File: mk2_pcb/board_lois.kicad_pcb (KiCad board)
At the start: 2 copper layers, 99 x 90 mm, 38 parts

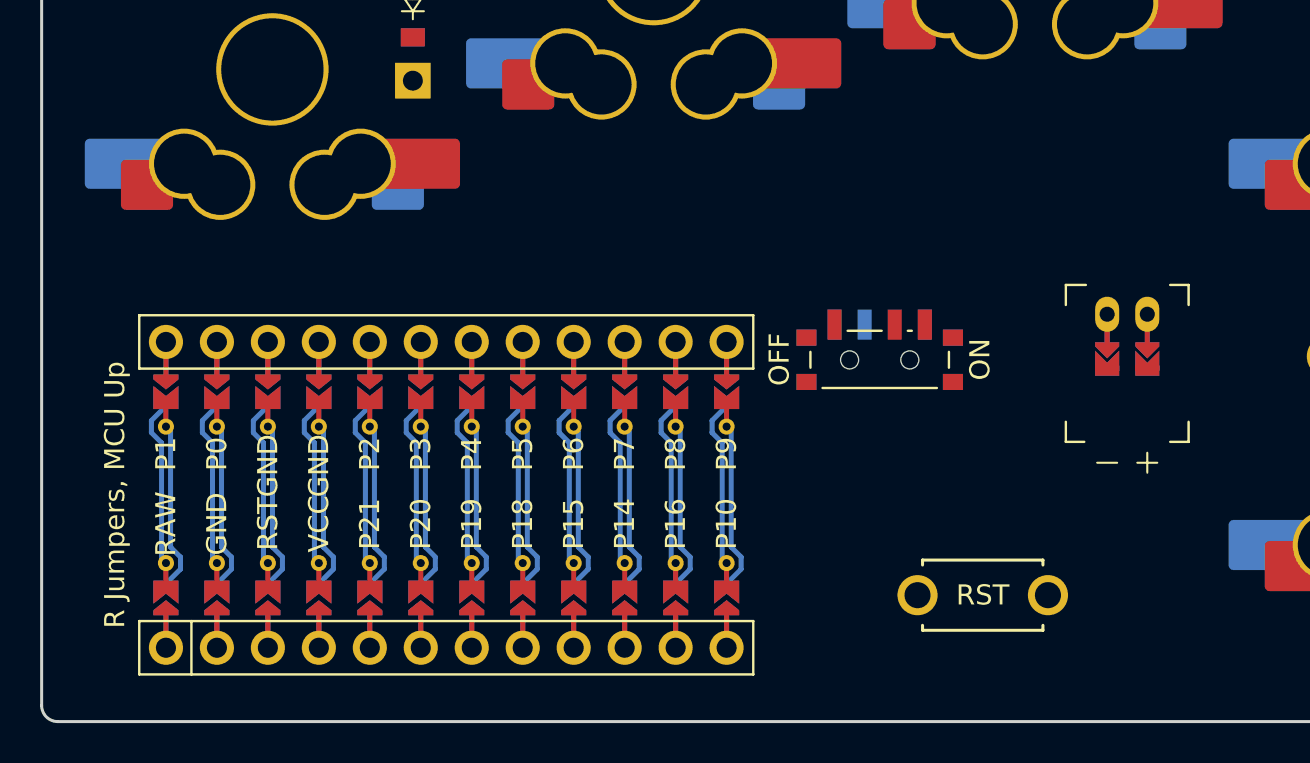
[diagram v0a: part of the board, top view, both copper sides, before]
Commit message: 19mm update
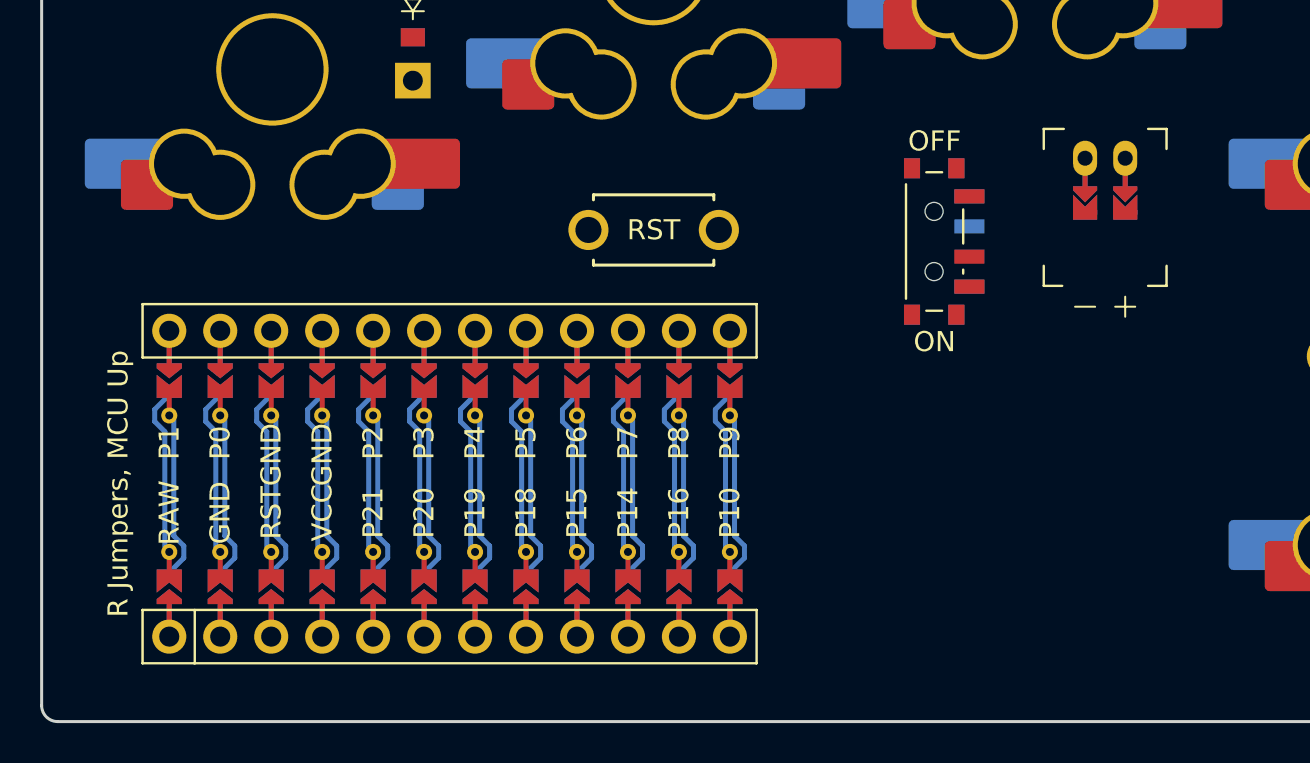
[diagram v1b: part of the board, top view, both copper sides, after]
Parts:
- moved RST1 24.5 mm to (194.0, 164.0)
- moved JST1 7.85 mm to (216.5, 160.4)
- moved PWR1 6.48 mm to (208.0, 164.6), turned to 180 degrees
- moved MCU1 0.58 mm to (182.6, 176.6)
